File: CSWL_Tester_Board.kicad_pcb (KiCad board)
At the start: 2 copper layers, 125.5 x 98 mm, 180 parts, among them J1 DB9_Female ID09S33E4GV00LF, J10 Conn_01x03_Male, J11 Conn_01x02, J12 Conn_01x03, J13 Conn_01x02, J14 Conn_01x04, J15 SPI1, J16 Conn_02x10_Odd_Even, J17 Conn_01x02, J18 Conn_01x02, J19 Conn_01x02, J2 Conn_01x04, J20 Conn_01x02, J21 Fix hole, J22 Conn_01x02, J23 Conn_01x03, J24 Conn_01x02, J25 USB_B_Micro, J26 Conn_01x04, J27 Conn_01x10, J28 Fix hole, J29 Fix hole, J3 Conn_01x04, J30 Fix hole, J31 Conn_Coaxial_Power, J4 Conn_01x04, J5 DB9_Female ID09S33E4GV00LF, J6 Conn_01x04, J7 Conn_01x04, J8 DB9_Female ID09S33E4GV00LF, J9 Conn_Coaxial_Power, K1 G6SU-2 DC5, K2 G6SU-2 DC5, K3 G6SU-2 DC5, K4 G6SU-2 DC5, K5 G6SU-2 DC5, Q1 DMG2301L, Q10 2N7002LT1G, Q11 2N7002LT1G, Q12 DMG2301L, Q13 2N7002LT1G, Q14 DMG2301L, Q2 DMG2301L, Q3 DMG2301L, Q4 2N7002LT1G, Q5 2N7002LT1G, Q6 2N7002LT1G, Q7 DMG2301L, Q8 DMG2301L, Q9 2N7002LT1G, U1 MAX3221EIPW, U10 EL817-S1-A (NC), U2 STM32F103RCT6, U3 MAX3221EIPW, U4 MCP1700T-3302E_TT, U5 MAX3221EIPW, U6 EL817-S1-A (NC), U7 EL817-S1-A (NC), U8 EL817-S1-A (NC), U9 EL817-S1-A (NC), Y1 Crystal_GND24

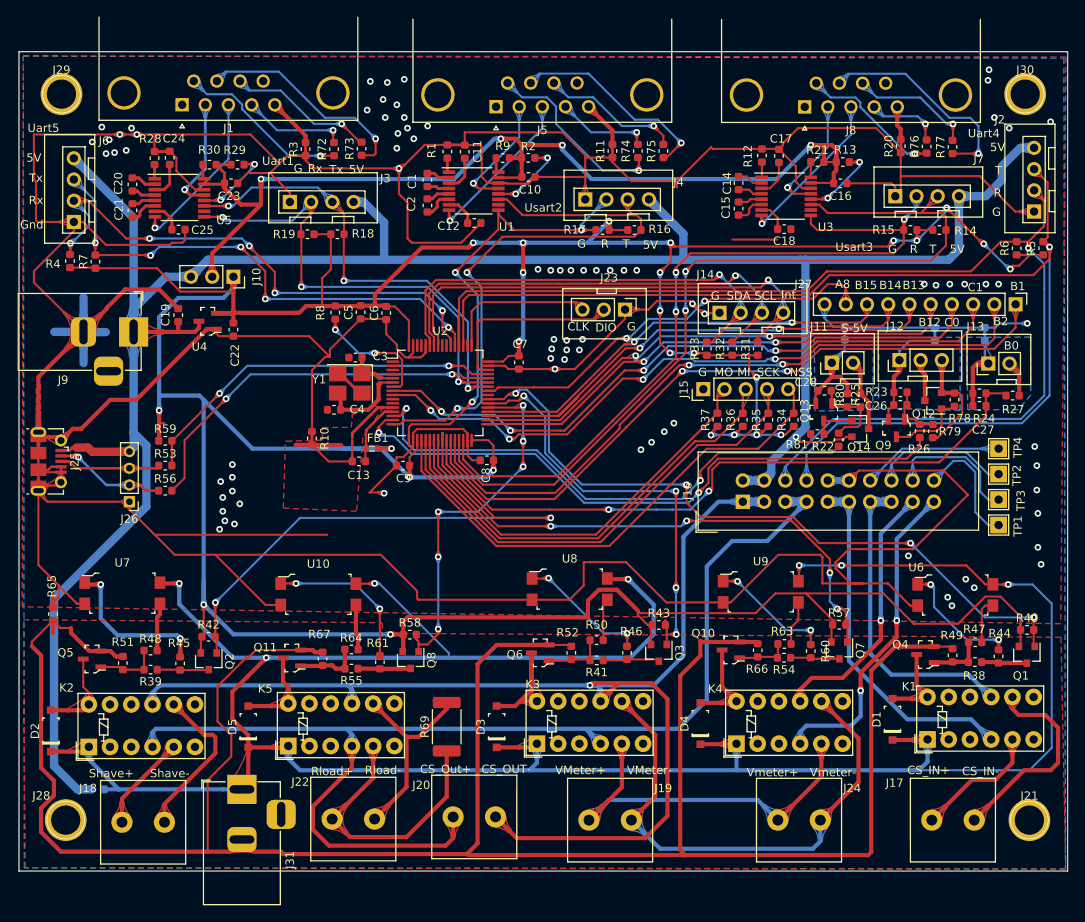
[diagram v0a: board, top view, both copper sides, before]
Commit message: Ruan: add treadrop
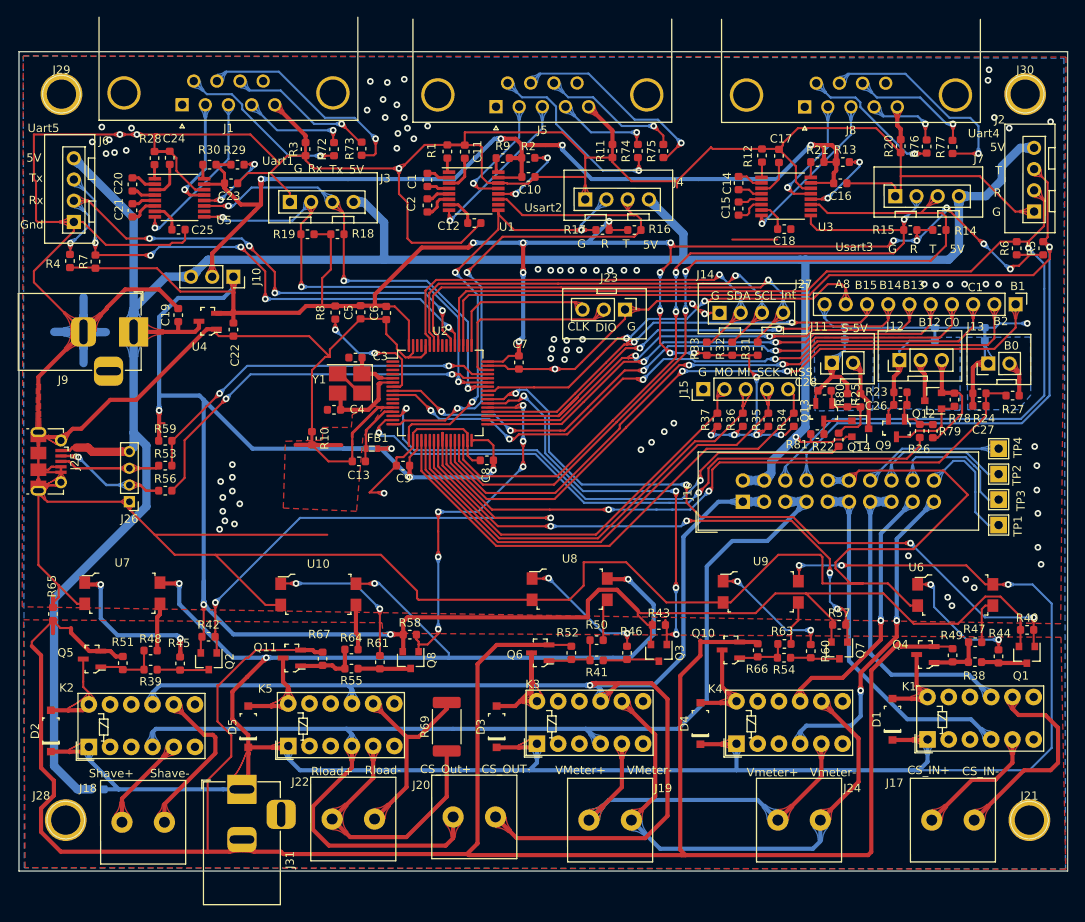
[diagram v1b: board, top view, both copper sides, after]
